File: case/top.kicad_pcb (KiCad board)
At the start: 2 copper layers, 135 x 95.7 mm, 25 parts, among them SW1 SW_PUSH, SW10 SW_PUSH, SW11 SW_PUSH, SW12 SW_PUSH, SW13 SW_PUSH, SW14 SW_PUSH, SW15 SW_PUSH, SW16 SW_PUSH, SW17 SW_PUSH, SW18 SW_PUSH, SW19 SW_PUSH, SW2 SW_PUSH, SW20 SW_PUSH, SW3 SW_PUSH, SW4 SW_PUSH, SW5 SW_PUSH, SW6 SW_PUSH, SW7 SW_PUSH, SW8 SW_PUSH, SW9 SW_PUSH

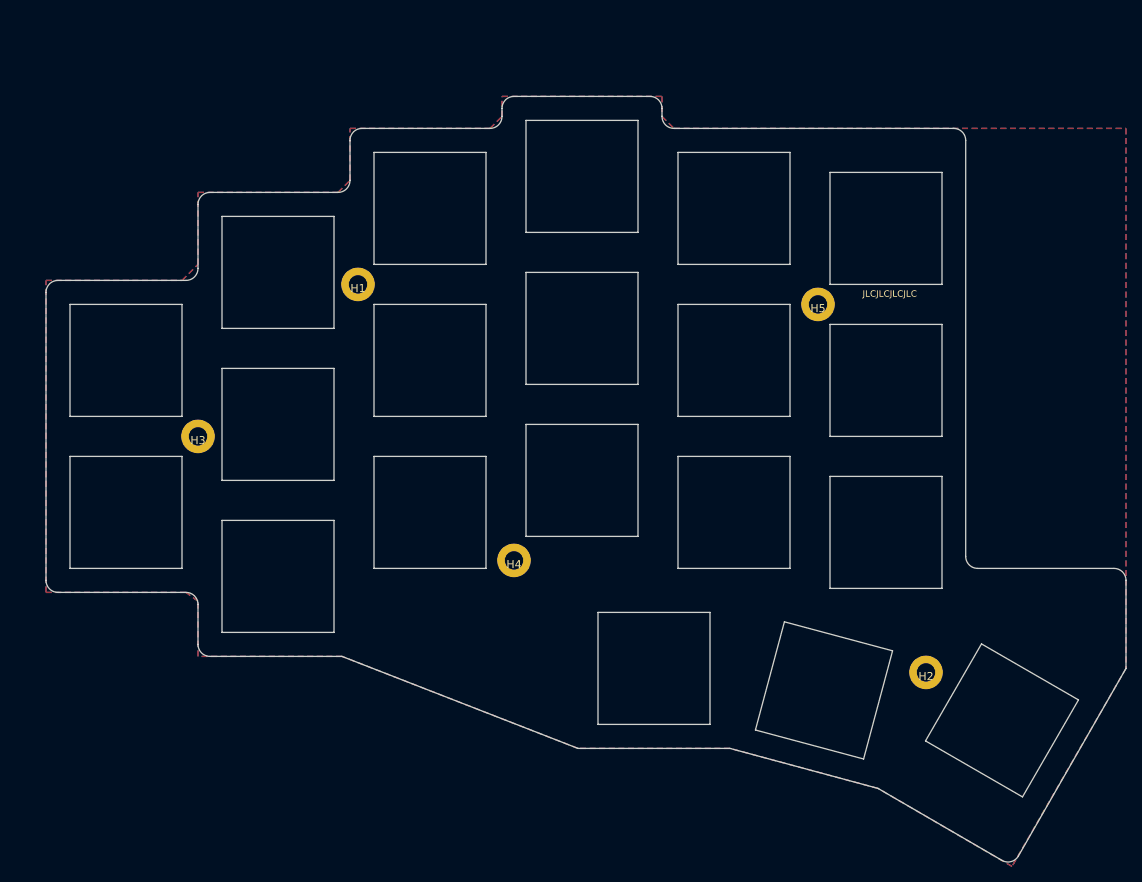
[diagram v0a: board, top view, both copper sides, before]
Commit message: update case files
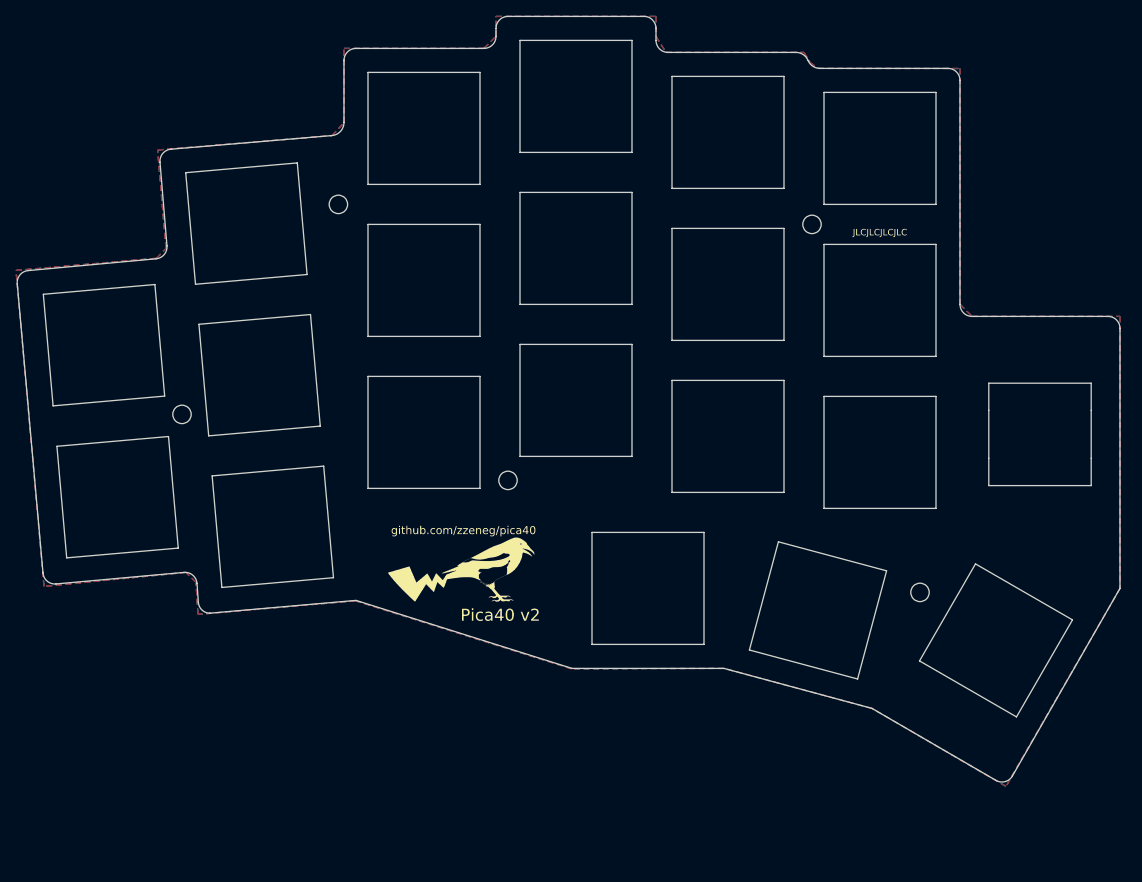
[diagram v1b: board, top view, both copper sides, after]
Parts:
- added G***: LOGO, pica:logo_mirror, F.Cu at (121.8, 112.1)
- added G***: LOGO, pica:logo, B.Cu at (121.8, 112.1)
- added RE1: RotaryEncoder_Switch, pica:EC11_Hole, F.Cu at (193.0, 95.2)
- H1, H2, H3, H4, H5: footprint kbd:M2_Hole_TH -> kbd:thread_m2
- moved H1 10.3 mm to (105.3, 66.5)
- moved H2 10.0 mm to (178.0, 115.0)
- moved H4 10.0 mm to (126.5, 101.0)
- moved H5 10.0 mm to (164.5, 69.0)
- moved SW10 10.0 mm to (173.0, 78.5)
- moved SW12 10.0 mm to (116.0, 95.0)
- moved SW13 10.0 mm to (135.0, 91.0)
- moved SW15 10.0 mm to (173.0, 97.5)
- moved SW18 10.0 mm to (144.0, 114.5)
- moved SW19 10.0 mm to (165.2, 117.2)
- moved SW2 10.0 mm to (116.0, 57.0)
- moved SW20 10.0 mm to (187.5, 121.0)
- moved SW3 10.0 mm to (135.0, 53.0)
- moved SW5 10.0 mm to (173.0, 59.5)
- moved SW7 10.0 mm to (116.0, 76.0)
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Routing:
- net empty: vias 0 -> 1
- added copper zone on B.Cu, net empty
- added copper zone on F.Cu, net empty
- removed copper zone on B.Cu, net (none)
- removed copper zone on F.Cu, net (none)
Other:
- board size 135 x 95.7 mm -> 137.8 x 95.7 mm
- board text added: "Pica40 v2"
- board text added: "github.com/zzeneg/pica40"
